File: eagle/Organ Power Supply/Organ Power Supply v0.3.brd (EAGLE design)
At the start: 58 x 45 mm, 22 parts, among them J1 PJ-102A, J10 CRESCENDO PEDAL, J11 POWER SWITCH, J2 USB-B, J3 54819-0519, J4 CHOIR MANUAL, J5 GREAT MANUAL, J6 SWELL MANUAL, J8 VOLUME PEDAL, J9 EXPRESSION PEDAL, U1 AP7361, U2 LM2940

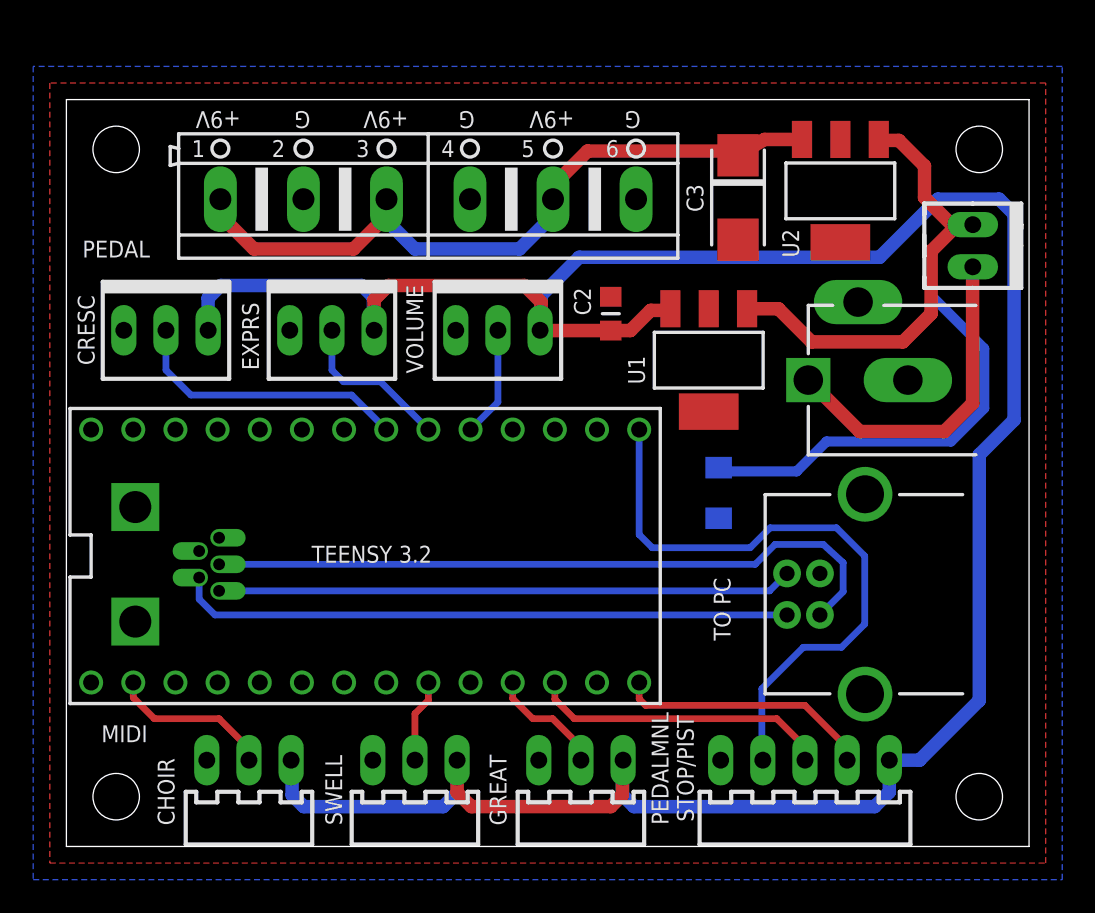
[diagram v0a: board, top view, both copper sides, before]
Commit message: Update eagle repos
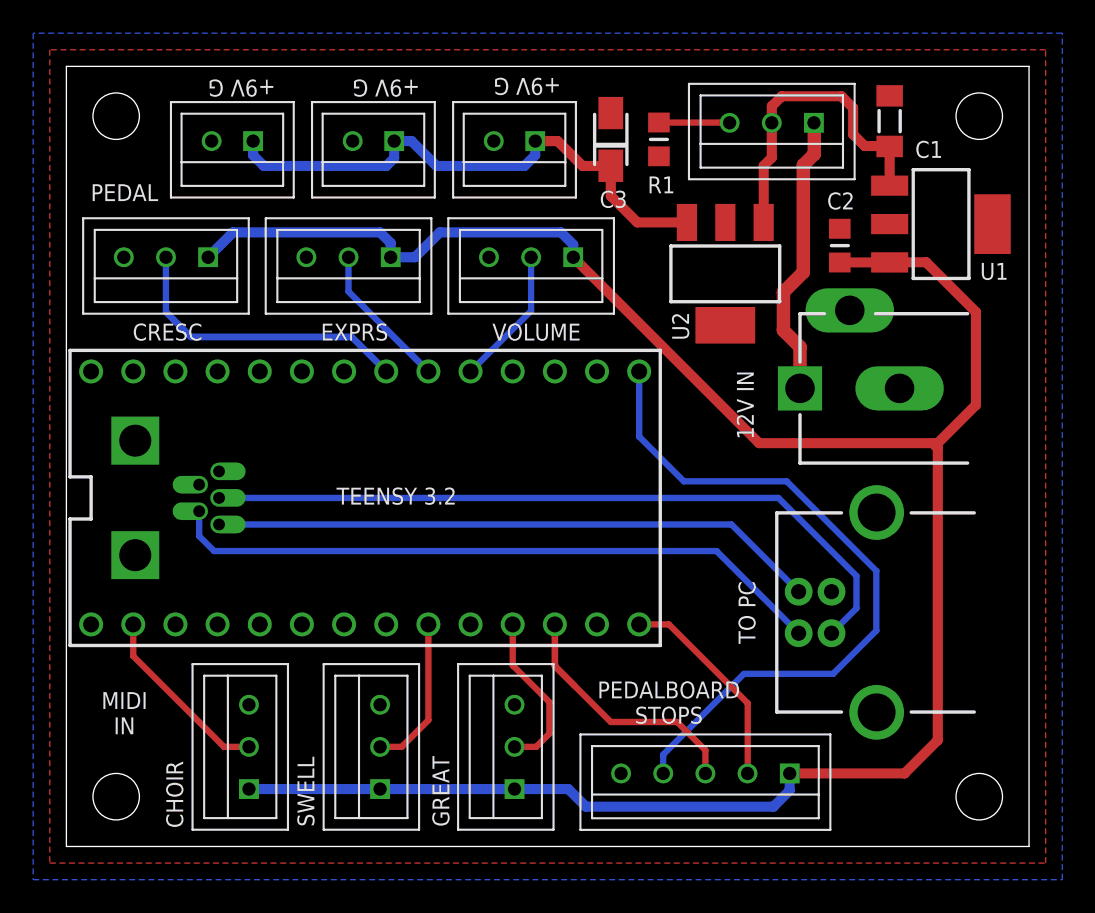
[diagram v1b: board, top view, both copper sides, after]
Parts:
- removed J10: CRESCENDO PEDAL, con-molex:6410-03
- removed J11: POWER SWITCH, con-molex:6410-02
- removed J4: CHOIR MANUAL, con-molex:7395-03
- removed J5: GREAT MANUAL, con-molex:7395-03
- removed J6: SWELL MANUAL, con-molex:7395-03
- removed J7: (no value), con-molex:7395-05
- removed J8: VOLUME PEDAL, con-molex:6410-03
- removed J9: EXPRESSION PEDAL, con-molex:6410-03
- added R1: 350R, rc-master-smd:R0805MP
- added X10: (no value), con-jst-xh:B5B-XH
- added X11: POWER SW, con-jst-xh:B3B-XH
- added X2, X3: B2B-XH, jdc:B2B-XH-A
- added X4: VOLUME PEDAL, con-jst-xh:B3B-XH
- added X5: EXPRESSION PEDAL, con-jst-xh:B3B-XH
- added X6: CRESCENDO PEDAL, con-jst-xh:B3B-XH
- added X7: CHOIR MANUAL, con-jst-xh:B3B-XH
- added X8: SWELL MANUAL, con-jst-xh:B3B-XH
- added X9: GREAT MANUAL, con-jst-xh:B3B-XH
- C1: value 1.0uF -> 6.8uF
- C2: value 0.1uF -> 10uF
- C3: device rc-master:C6032-28R/T -> rc-master:C3216-18R/T
- U1: value AP7361 -> SPX3940
- X1: value (none) -> B2B-XH; device con-ptr500:AK500/6 -> jdc:B2B-XH-A
- moved C1 24.7 mm to (49.6, 43.7), flipped to the top, turned to 270 degrees
- moved U1 16.2 mm to (52.7, 37.5), turned to 270 degrees
- moved C2 14.4 mm to (46.6, 36.2)
- moved U2 8.55 mm to (39.7, 34.5)
- moved C3 8.43 mm to (32.8, 42.6), turned to 270 degrees
- moved X1 6.27 mm to (27.0, 42.5), turned to 180 degrees
- moved J3 4.00 mm to (9.20, 21.0)
- moved B1 3.50 mm to (18.0, 21.0)
- moved HOLE2 2.00 mm to (3.00, 44.0)
- moved HOLE4 2.00 mm to (55.0, 44.0)
- moved J2 1.30 mm to (46.1, 14.1)
- moved J1 0.71 mm to (44.2, 27.6)
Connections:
- new net N$3: R1.1, X11.P$3
- net +3V3: now also X10.P$1, X4.P$1, X5.P$1, X6.P$1, X7.P$1, X8.P$1, X9.P$1; no longer J10.1, J4.1, J5.1, J6.1, J7.1, J8.1, J9.1
- net +9V: now also X1.P$1, X2.P$1, X3.P$1; no longer X1.1, X1.3, X1.5
- net A3: now also X4.P$2; no longer J8.2
- net A4: now also X5.P$2; no longer J9.2
- net A5: now also X6.P$2; no longer J10.2
- net CS: now also X10.P$3; no longer J7.3
- net GND: now also R1.2, X1.P$2, X10.P$5, X2.P$2, X3.P$2, X4.P$3, X5.P$3, X6.P$3, X7.P$3, X8.P$3, X9.P$3; no longer J10.3, J4.3, J5.3, J6.3, J7.5, J8.3, J9.3, X1.2, X1.4, X1.6
- net MISO: now also X10.P$2; no longer J7.2
- net N$2: now also X11.P$1; no longer J11.1
- net RX1: now also X7.P$2; no longer J4.2
- net RX2: now also X9.P$2; no longer J5.2
- net RX3: now also X8.P$2; no longer J6.2
- net SCK: now also X10.P$4; no longer J7.4
- net VEXT: now also X11.P$2; no longer J11.2
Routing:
- net VEXT: track 59.1 -> 19.1 mm
- net +3V3: track 157.9 -> 132.6 mm
- net +9V: track 45.3 -> 33.3 mm
- net SCK: track 37.7 -> 42.2 mm
- net RX3: track 5.02 -> 9.35 mm
- net N$3: track 0.00 -> 4.26 mm
- net CS: track 18.1 -> 15.1 mm
- net N$9: track 37.1 -> 40.0 mm
- net N$2: track 20.1 -> 17.2 mm
- net RX2: track 7.09 -> 9.93 mm
- net MISO: track 15.5 -> 12.7 mm
- net N$8: track 42.3 -> 44.4 mm
- net N$1: track 34.7 -> 36.6 mm
- net A3: track 6.66 -> 8.39 mm
- net RX1: track 9.85 -> 11.1 mm
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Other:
- board size 58 x 45 mm -> 58 x 47 mm
- board text added: "+9V G"
- board text added: "12V IN"
- board text added: "9V"
- board text added: "LED-"
- board text added: "MIDI IN"
- board text added: "PEDALBOARD STOPS"
- board text added: "VIN"
- board text added: "VSW"
- board text removed: "+9V"
- board text removed: "G"
- board text removed: "MIDI"
- board text removed: "PEDALMNL STOP/PIST"
